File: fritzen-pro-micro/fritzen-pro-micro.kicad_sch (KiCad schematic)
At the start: 3 parts, among them J1 Conn_01x12_Pin, J2 Conn_01x12_Pin, J3 Conn_01x22_Pin

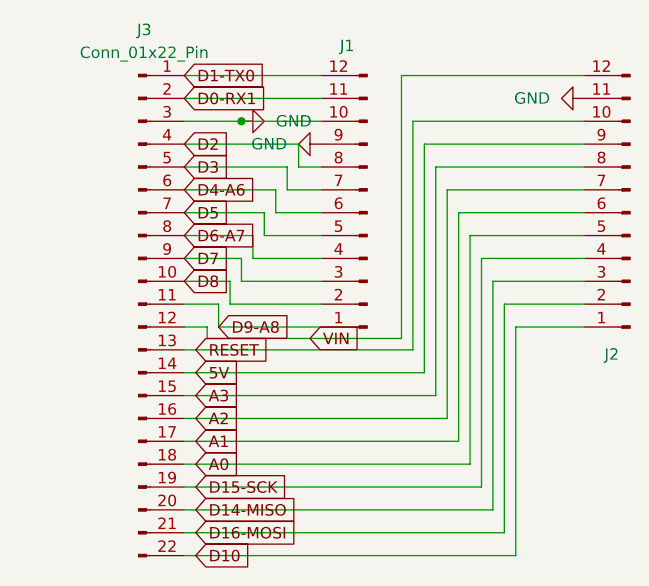
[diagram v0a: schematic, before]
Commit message: Started layouting
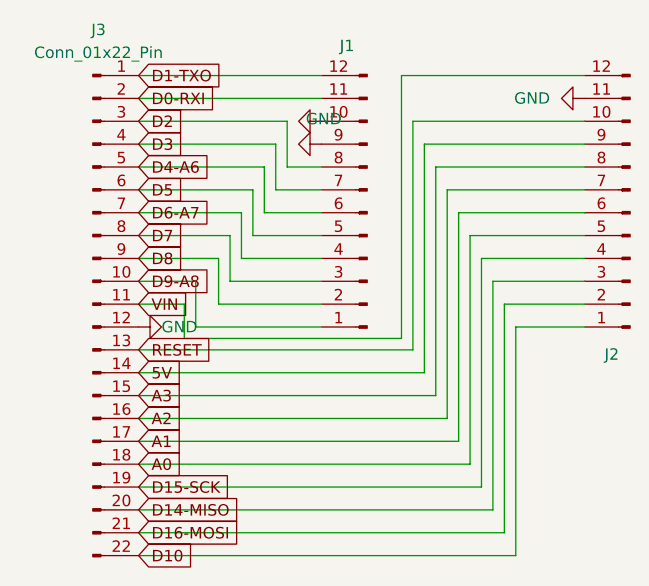
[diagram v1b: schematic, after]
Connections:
- net D2: now also J3.3 (Pin_3); no longer J3.4 (Pin_4)
- net D3: now also J3.4 (Pin_4); no longer J3.5 (Pin_5)
- net D4-A6: now also J3.5 (Pin_5); no longer J3.6 (Pin_6)
- net D5: now also J3.6 (Pin_6); no longer J3.7 (Pin_7)
- net D6-A7: now also J3.7 (Pin_7); no longer J3.8 (Pin_8)
- net D7: now also J3.8 (Pin_8); no longer J3.9 (Pin_9)
- net D8: now also J3.9 (Pin_9); no longer J3.10 (Pin_10)
- net D9-A8: now also J3.10 (Pin_10); no longer J3.11 (Pin_11)
- net GND: now also J3.12 (Pin_12); no longer J3.3 (Pin_3)
- net VIN: now also J3.11 (Pin_11); no longer J3.12 (Pin_12)
- net D0-RX1 renamed D0-RXI
- net D1-TX0 renamed D1-TXO
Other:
- moved on the sheet: J3
